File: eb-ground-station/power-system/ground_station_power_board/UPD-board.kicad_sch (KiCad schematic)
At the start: 101 parts, among them J1 Conn_01x04, J10 PI 1827486, J11 PC 1720806, J12 Conn_02x02_Odd_Even, J13 Conn_01x05, J14 Conn_01x04, J2 Conn_01x03, J3 Conn_01x03, J4 Conn_01x03, J5 Conn_01x03, J6 Conn_01x03, J7 PI 1924143, J8 PI 1827923, J9 PI 1827486, Q21 SUD50P08-25L-E3, Q22 SUD50P08-25L-E3, U1 MAX7310, U2 MAX7310, U3 MAX7310, U4 ADT7410TRZ, U5 ADS1115IDGS, U6 UA78M33, U7 U_RasPi_40pin

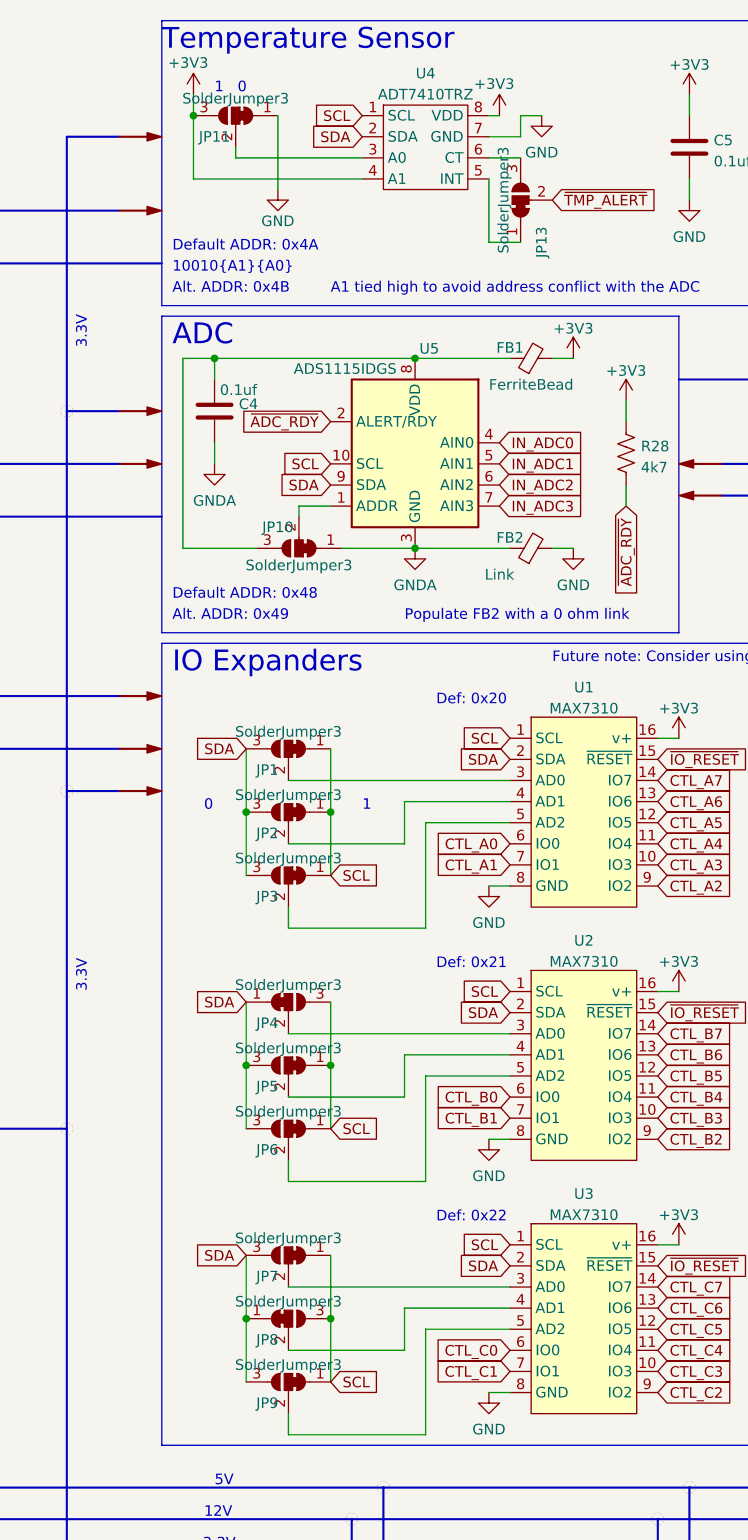
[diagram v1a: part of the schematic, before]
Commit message: updated board changes for bom
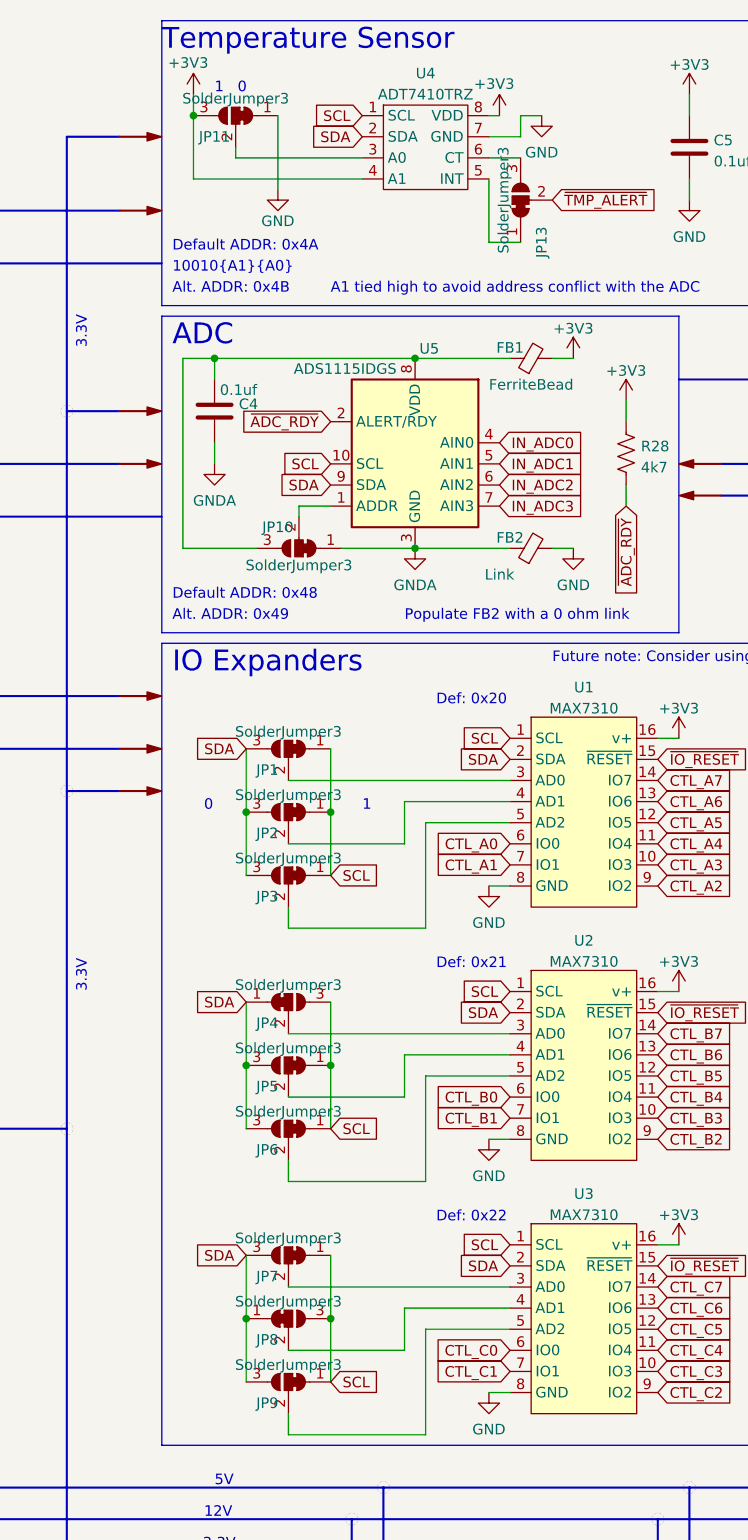
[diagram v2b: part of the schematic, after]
